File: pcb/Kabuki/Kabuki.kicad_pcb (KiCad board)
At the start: 2 copper layers, 70 x 40 mm, 14 parts, among them J1 NC3FAHL1, J2 NC3MAHR, J3 Solenoide, Q1 FQD18N20V2TM, Q2 FQD18N20V2TM, U1 IX4428N

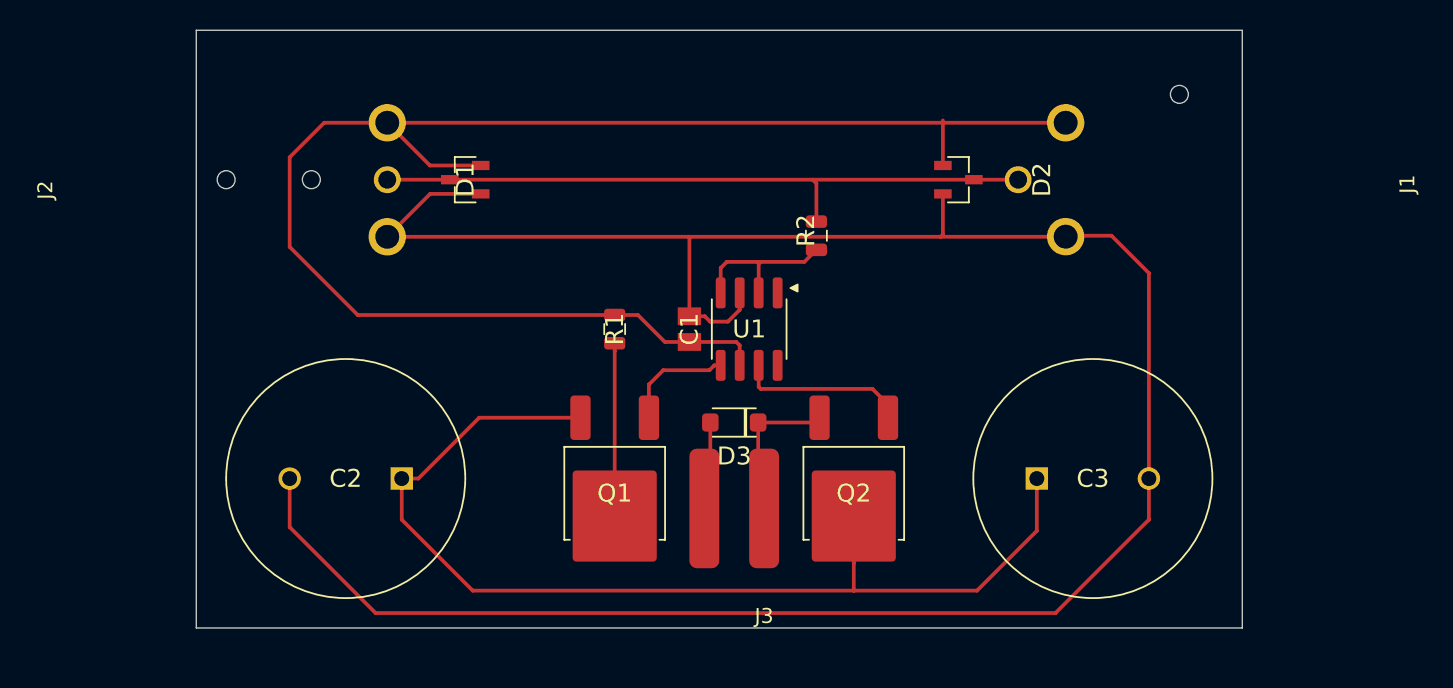
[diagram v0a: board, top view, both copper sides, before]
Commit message: update
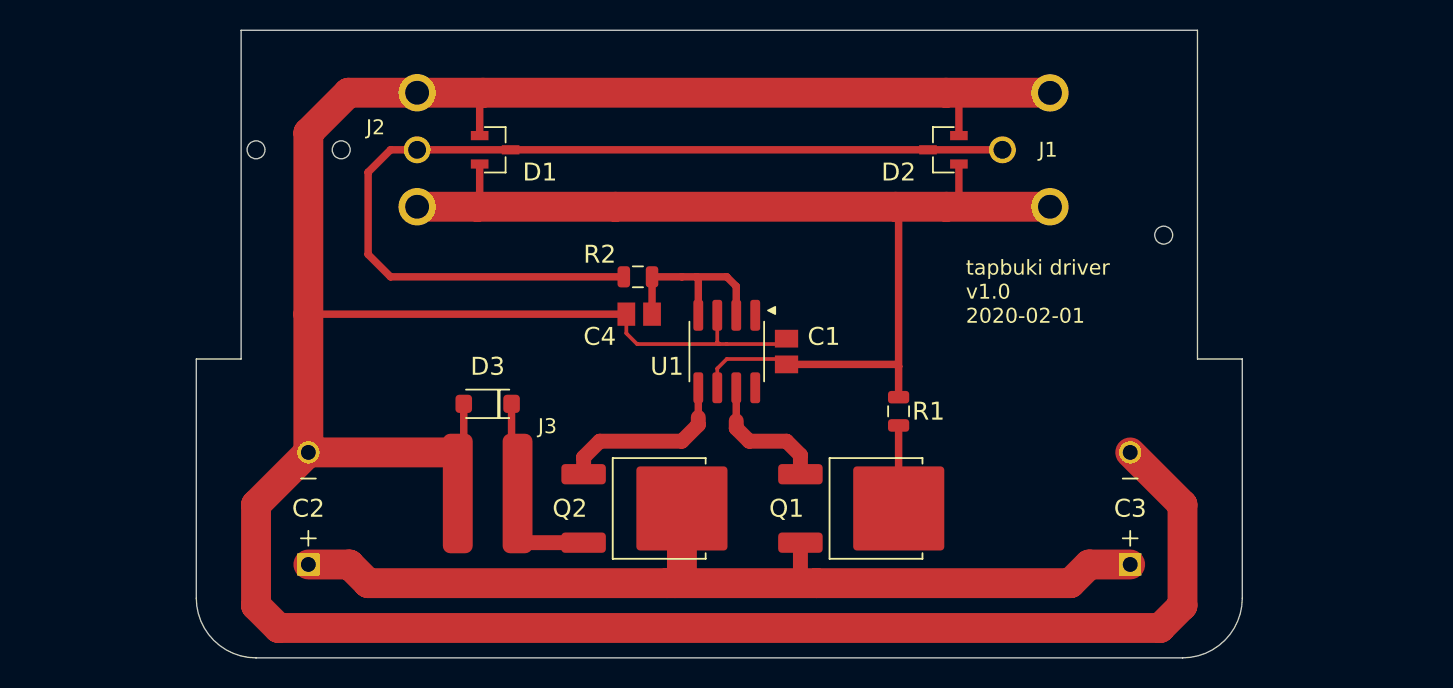
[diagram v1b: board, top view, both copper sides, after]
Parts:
- added C4: capcer0805, Kabuki:CAP0805, F.Cu at (129.6, 69.0)
- C2, C3, J1, J2: moved to B.Cu
- moved R1 19.8 mm to (147.0, 75.5)
- moved Q1 16.6 mm to (144.5, 82.0), turned to 270 degrees
- moved D3 16.5 mm to (119.5, 75.0)
- moved J3 16.5 mm to (121.5, 81.0)
- moved Q2 14.2 mm to (130.0, 82.0), turned to 270 degrees
- moved R2 12.3 mm to (129.6, 66.5), turned to 180 degrees
- moved C1 6.67 mm to (139.5, 71.5)
- moved C2 3.20 mm to (107.5, 82.0), turned to 90 degrees
- moved C3 3.20 mm to (162.5, 82.0), turned to 90 degrees
- moved D1 2.83 mm to (120.0, 58.0), turned to 270 degrees
- moved J2 2.83 mm to (97.0, 58.0), turned to 270 degrees
- moved J1 2.26 mm to (173.0, 58.0), turned to 90 degrees
- moved D2 2.24 mm to (150.0, 58.0), turned to 90 degrees
- moved U1 2.12 mm to (135.5, 71.5)
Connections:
- U1 pad 5: Net-(Q1-Pad1) -> Net-(Q2-Pad1)
- U1 pad 7: Net-(Q2-Pad1) -> Net-(Q1-Pad1)
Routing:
- net GND: track 160.9 -> 219.4 mm
- net +5VD: track 103.5 -> 75.2 mm
- net Net-(D1-Pad3): track 45.1 -> 66.3 mm
- net Net-(C2-Pad1): track 71.0 -> 64.1 mm
- net Net-(Q1-Pad3): track 11.6 -> 5.56 mm
- net Net-(D3-PadC): track 10.2 -> 13.7 mm
- net Net-(C4-Pad2): track 10.7 -> 13.0 mm
- net Net-(Q1-Pad1): track 7.56 -> 9.03 mm
- net Net-(Q2-Pad1): track 11.5 -> 12.2 mm
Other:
- board size 70 x 40 mm -> 70 x 42 mm
- board text added: "tapbuki driver v1.0 2020-02-01"
